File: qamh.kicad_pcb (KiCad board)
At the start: 2 copper layers, 40.3 x 128.5 mm, 17 parts, among them J1 Eurorack_Power_16pin_Shrouded, J2 OUTPUT, J3 INPUT 1, J4 INPUT 2, J5 INPUT 3

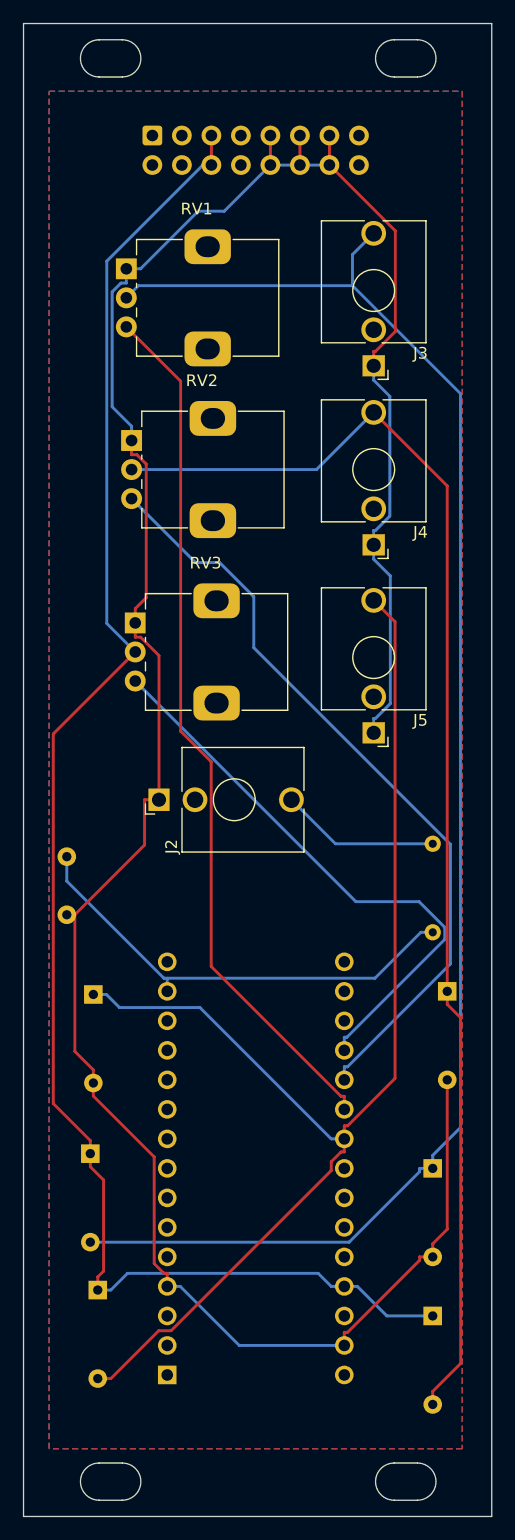
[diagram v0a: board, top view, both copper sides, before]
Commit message: fix
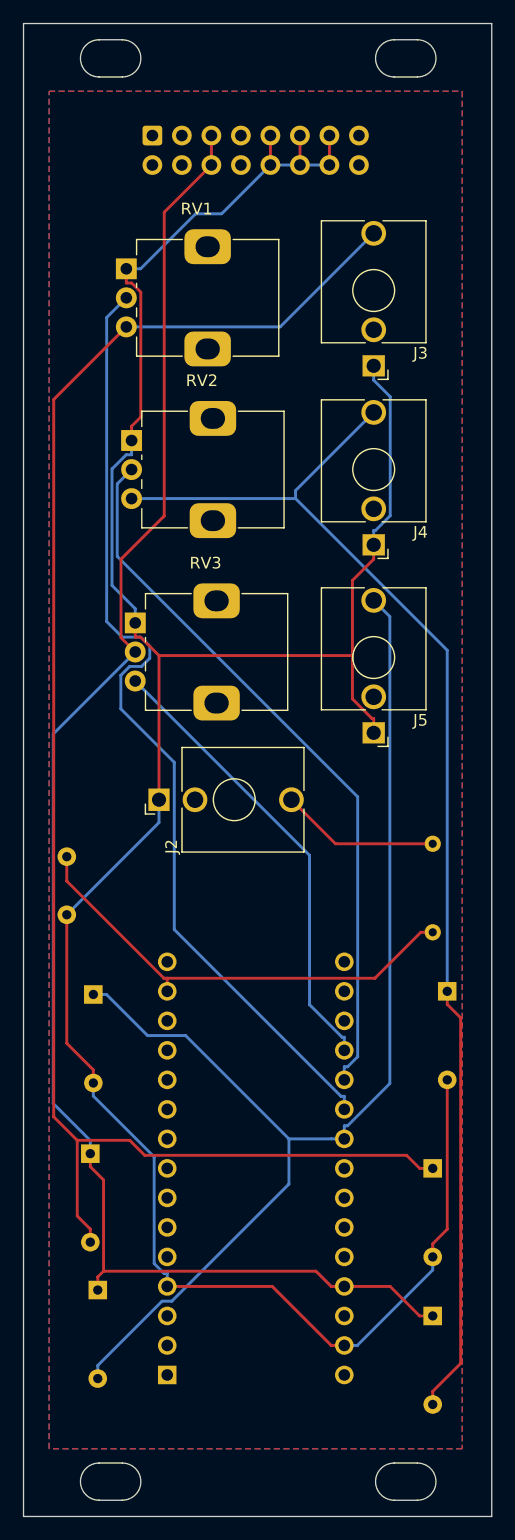
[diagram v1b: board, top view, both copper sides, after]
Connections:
- A1 pad 21: Net-(A1-Pad21) -> Net-(RV1-Pad2)
- D5 pad 2: Net-(D5-Pad2) -> Net-(RV2-Pad3)
- D6 pad 1: Net-(D5-Pad2) -> Net-(RV2-Pad3)
- J4 pad T: Net-(D5-Pad2) -> Net-(RV2-Pad3)
- RV1 pad 2: Net-(D1-Pad2) -> Net-(RV1-Pad2)
- RV1 pad 3: Net-(A1-Pad21) -> Net-(D1-Pad2)
- RV2 pad 2: Net-(D5-Pad2) -> Net-(A1-Pad20)
- RV2 pad 3: Net-(A1-Pad20) -> Net-(RV2-Pad3)
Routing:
- net Net-(D5-Pad2): track 112.4 -> 0.00 mm
- net Net-(RV2-Pad3): track 0.00 -> 109.2 mm
- net Net-(RV1-Pad2): track 0.00 -> 82.8 mm
- net Net-(A1-Pad21): track 75.3 -> 0.00 mm
- net Net-(A1-Pad19): track 49.7 -> 39.4 mm
- net Net-(A1-Pad20): track 66.6 -> 62.3 mm
- net GND: track 227.3 -> 223.1 mm
- net Net-(A1-Pad22): track 106.7 -> 103.4 mm
- net +5V: track 140.4 -> 138.0 mm
- net Net-(D1-Pad2): track 138.2 -> 138.9 mm
